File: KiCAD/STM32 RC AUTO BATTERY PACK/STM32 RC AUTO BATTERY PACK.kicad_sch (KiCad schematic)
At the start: 4 parts

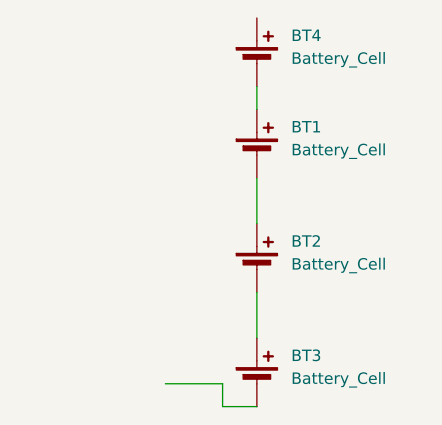
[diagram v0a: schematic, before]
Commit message: ,
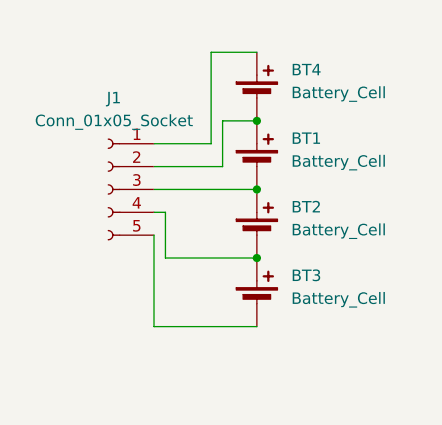
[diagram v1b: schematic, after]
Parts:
- added J1: Conn_01x05_Socket, Connector_JST:JST_XH_B5B-XH-A_1x05_P2.50mm_Vertical, symbol Connector:Conn_01x05_Socket
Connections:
- net at BT2.2 (-), BT3.1 (+): now also J1.4 (Pin_4)
- net at BT3.2 (-): now also J1.5 (Pin_5)
- net at BT1.2 (-), BT2.1 (+): now also J1.3 (Pin_3)
- net at BT4.1 (+): now also J1.1 (Pin_1)
- net at BT1.1 (+), BT4.2 (-): now also J1.2 (Pin_2)
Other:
- moved on the sheet: BT1, BT2, BT3, BT4
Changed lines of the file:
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@@
 	(generator_version "9.0")
 	(paper "A4")
-	(wire
-		(pts
-			(xy 121.92 63.5) (xy 121.92 68.58)
-		)
-		(stroke
-			(width 0)
-			(type default)
-		)
-	)
-	(wire
-		(pts
-			(xy 121.92 76.2) (xy 118.11 76.2)
-		)
-		(stroke
-			(width 0)
-			(type default)
-		)
-	)
-	(wire
-		(pts
-			(xy 118.11 73.66) (xy 111.76 73.66)
-		)
-		(stroke
-			(width 0)
-			(type default)
-		)
-	)
-	(wire
-		(pts
-			(xy 121.92 40.64) (xy 121.92 43.18)
-		)
-		(stroke
-			(width 0)
-			(type default)
-		)
-	)
-	(wire
-		(pts
-			(xy 121.92 50.8) (xy 121.92 55.88)
-		)
-		(stroke
-			(width 0)
-			(type default)
-		)
-	)
-	(wire
-		(pts
-			(xy 118.11 76.2) (xy 118.11 73.66)
+	(junction
+		(at 121.92 44.45)
+		(diameter 0)
+		(color 0 0 0 0)
+	)
+	(junction
+		(at 121.92 59.69)
+		(diameter 0)
+		(color 0 0 0 0)
+	)
+	(junction
+		(at 121.92 52.07)
+		(diameter 0)
+		(color 0 0 0 0)
+	)
+	(wire
+		(pts
+			(xy 121.92 67.31) (xy 110.49 67.31)
+		)
+		(stroke
+			(width 0)
+			(type default)
+		)
+	)
+	(wire
+		(pts
+			(xy 111.76 59.69) (xy 111.76 54.61)
+		)
+		(stroke
+			(width 0)
+			(type default)
+		)
+	)
+	(wire
+		(pts
+			(xy 110.49 57.15) (xy 110.49 67.31)
+		)
+		(stroke
+			(width 0)
+			(type default)
+		)
+	)
+	(wire
+		(pts
+			(xy 110.49 52.07) (xy 121.92 52.07)
+		)
+		(stroke
+			(width 0)
+			(type default)
+		)
+	)
+	(wire
+		(pts
+			(xy 121.92 59.69) (xy 111.76 59.69)
+		)
+		(stroke
+			(width 0)
+			(type default)
+		)
+	)
+	(wire
+		(pts
+			(xy 118.11 44.45) (xy 118.11 49.53)
+		)
+		(stroke
+			(width 0)
+			(type default)
+		)
+	)
+	(wire
+		(pts
+			(xy 121.92 44.45) (xy 118.11 44.45)
+		)
+		(stroke
+			(width 0)
+			(type default)
+		)
+	)
+	(wire
+		(pts
+			(xy 111.76 54.61) (xy 110.49 54.61)
+		)
+		(stroke
+			(width 0)
+			(type default)
+		)
+	)
+	(wire
+		(pts
+			(xy 118.11 49.53) (xy 110.49 49.53)
+		)
+		(stroke
+			(width 0)
+			(type default)
+		)
+	)
+	(wire
+		(pts
+			(xy 116.84 46.99) (xy 110.49 46.99)
+		)
+		(stroke
+			(width 0)
+			(type default)
+		)
+	)
+	(wire
+		(pts
+			(xy 116.84 36.83) (xy 116.84 46.99)
+		)
+		(stroke
+			(width 0)
+			(type default)
+		)
+	)
+	(wire
+		(pts
+			(xy 121.92 36.83) (xy 116.84 36.83)
 		)
 		(stroke
@@
 	(symbol
 		(lib_id "Device:Battery_Cell")
-		(at 121.92 73.66 0)
+		(at 121.92 64.77 0)
 		(unit 1)
 		(exclude_from_sim no)
@@
 		(fields_autoplaced yes)
 		(property "Reference" "BT3"
-			(at 125.73 70.5484 0)
+			(at 125.73 61.6584 0)
 			(effects
 				(font
@@
 		)
 		(property "Value" "Battery_Cell"
-			(at 125.73 73.0884 0)
+			(at 125.73 64.1984 0)
 			(effects
 				(font
@@
 		)
 		(property "Footprint" "Batteryholder:21700 laskakit battery holder"
-			(at 121.92 72.136 90)
+			(at 121.92 63.246 90)
 			(effects
 				(font
@@
 		)
 		(property "Datasheet" "~"
-			(at 121.92 72.136 90)
+			(at 121.92 63.246 90)
 			(effects
 				(font
@@
 		)
 		(property "Description" "Single-cell battery"
-			(at 121.92 73.66 0)
+			(at 121.92 64.77 0)
 			(effects
 				(font
@@
 	(symbol
 		(lib_id "Device:Battery_Cell")
-		(at 121.92 60.96 0)
+		(at 121.92 57.15 0)
 		(unit 1)
 		(exclude_from_sim no)
@@
 		(fields_autoplaced yes)
 		(property "Reference" "BT2"
-			(at 125.73 57.8484 0)
+			(at 125.73 54.0384 0)
 			(effects
 				(font
@@
 		)
 		(property "Value" "Battery_Cell"
-			(at 125.73 60.3884 0)
+			(at 125.73 56.5784 0)
 			(effects
 				(font
@@
 		)
 		(property "Footprint" "Batteryholder:21700 laskakit battery holder"
-			(at 121.92 59.436 90)
+			(at 121.92 55.626 90)
 			(effects
 				(font
@@
 		)
 		(property "Datasheet" "~"
-			(at 121.92 59.436 90)
+			(at 121.92 55.626 90)
 			(effects
 				(font
@@
 		)
 		(property "Description" "Single-cell battery"
-			(at 121.92 60.96 0)
+			(at 121.92 57.15 0)
 			(effects
 				(font
@@
 	(symbol
 		(lib_id "Device:Battery_Cell")
-		(at 121.92 38.1 0)
+		(at 121.92 41.91 0)
 		(unit 1)
 		(exclude_from_sim no)
@@
 		(fields_autoplaced yes)
 		(property "Reference" "BT4"
-			(at 125.73 34.9884 0)
+			(at 125.73 38.7984 0)
 			(effects
 				(font
@@
 		)
 		(property "Value" "Battery_Cell"
-			(at 125.73 37.5284 0)
+			(at 125.73 41.3384 0)
 			(effects
 				(font
@@
 		)
 		(property "Footprint" "Batteryholder:21700 laskakit battery holder"
-			(at 121.92 36.576 90)
+			(at 121.92 40.386 90)
 			(effects
 				(font
@@
 		)
 		(property "Datasheet" "~"
-			(at 121.92 36.576 90)
+			(at 121.92 40.386 90)
 			(effects
 				(font
@@
 		)
 		(property "Description" "Single-cell battery"
-			(at 121.92 38.1 0)
+			(at 121.92 41.91 0)
 			(effects
 				(font
@@
 	(symbol
 		(lib_id "Device:Battery_Cell")
-		(at 121.92 48.26 0)
+		(at 121.92 49.53 0)
 		(unit 1)
 		(exclude_from_sim no)
@@
 		(fields_autoplaced yes)
 		(property "Reference" "BT1"
-			(at 125.73 45.1484 0)
+			(at 125.73 46.4184 0)
 			(effects
 				(font
@@
 		)
 		(property "Value" "Battery_Cell"
-			(at 125.73 47.6884 0)
+			(at 125.73 48.9584 0)
 			(effects
 				(font
@@
 		)
 		(property "Footprint" "Batteryholder:21700 laskakit battery holder"
-			(at 121.92 46.736 90)
+			(at 121.92 48.006 90)
 			(effects
 				(font
@@
 		)
 		(property "Datasheet" "~"
-			(at 121.92 46.736 90)
+			(at 121.92 48.006 90)
 			(effects
 				(font
@@
 		)
 		(property "Description" "Single-cell battery"
-			(at 121.92 48.26 0)
+			(at 121.92 49.53 0)
 			(effects
 				(font
@@
 					(unit 1)
 				)
+			)
+		)
+	)
+	(symbol
+		(lib_id "Connector:Conn_01x05_Socket")
+		(at 105.41 52.07 0)
+		(mirror y)
+		(unit 1)
+		(exclude_from_sim no)
+		(in_bom yes)
+		(on_board yes)
+		(dnp no)
+		(fields_autoplaced yes)
+		(property "Reference" "J1"
+			(at 106.045 41.91 0)
+			(effects
+				(font
+					(size 1.27 1.27)
+				)
+			)
+		)
+		(property "Value" "Conn_01x05_Socket"
+			(at 106.045 44.45 0)
+			(effects
+				(font
+					(size 1.27 1.27)
+				)
+			)
+		)
+		(property "Footprint" "Connector_JST:JST_XH_B5B-XH-A_1x05_P2.50mm_Vertical"
+			(at 105.41 52.07 0)
+			(effects
+				(font
+					(size 1.27 1.27)
+				)
+				(hide yes)
+			)
+		)
+		(property "Datasheet" "~"
+			(at 105.41 52.07 0)
+			(effects
+				(font
+					(size 1.27 1.27)
+				)
+				(hide yes)
+			)
+		)
+		(property "Description" "Generic connector, single row, 01x05, script generated"
+			(at 105.41 52.07 0)
+			(effects
+				(font
+					(size 1.27 1.27)
+				)
+				(hide yes)
+			)
+		)
+		(pin "3"
+		)
+		(pin "1"
+		)
+		(pin "2"
+		)
+		(pin "4"
+		)
+		(pin "5"
+		)
+		(instances
+			(project ""
+				(path "/b1f9147f-46b9-47b9-837a-c3ed0b7f7b76"
+					(reference "J1")
+					(unit 1)
+				)
